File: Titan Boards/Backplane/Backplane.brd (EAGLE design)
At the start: 209.6 x 76.2 mm, 20 parts

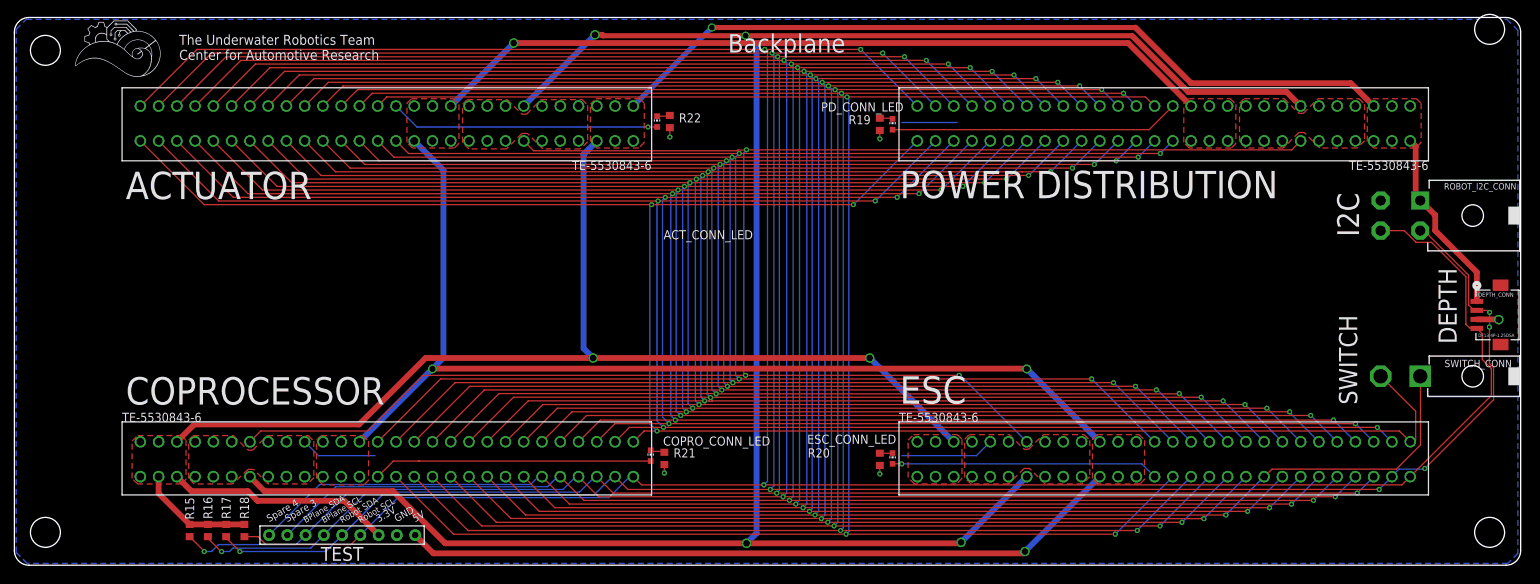
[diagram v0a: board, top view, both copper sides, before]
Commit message: final backplane fixes
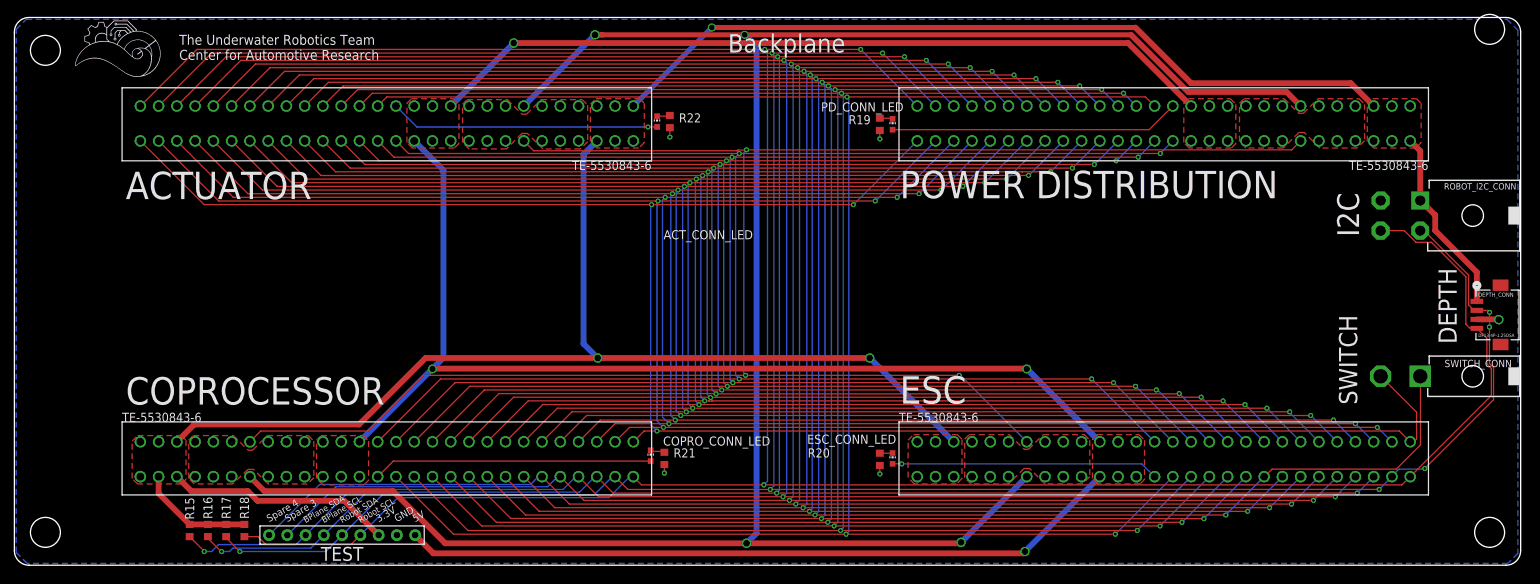
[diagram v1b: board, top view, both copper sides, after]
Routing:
- net GND: track 39.3 -> 7.92 mm
- net ROBOT_SCL: track 393.9 -> 392.1 mm
